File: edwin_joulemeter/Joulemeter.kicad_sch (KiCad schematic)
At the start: 57 parts, among them J1 XT60-M, J2 22035035, J3 22035035, J4 XT60-M, U1 INA240A3PWR, U3 MCP6286T-E/OT, U4 PADS131M04QPWRQ1

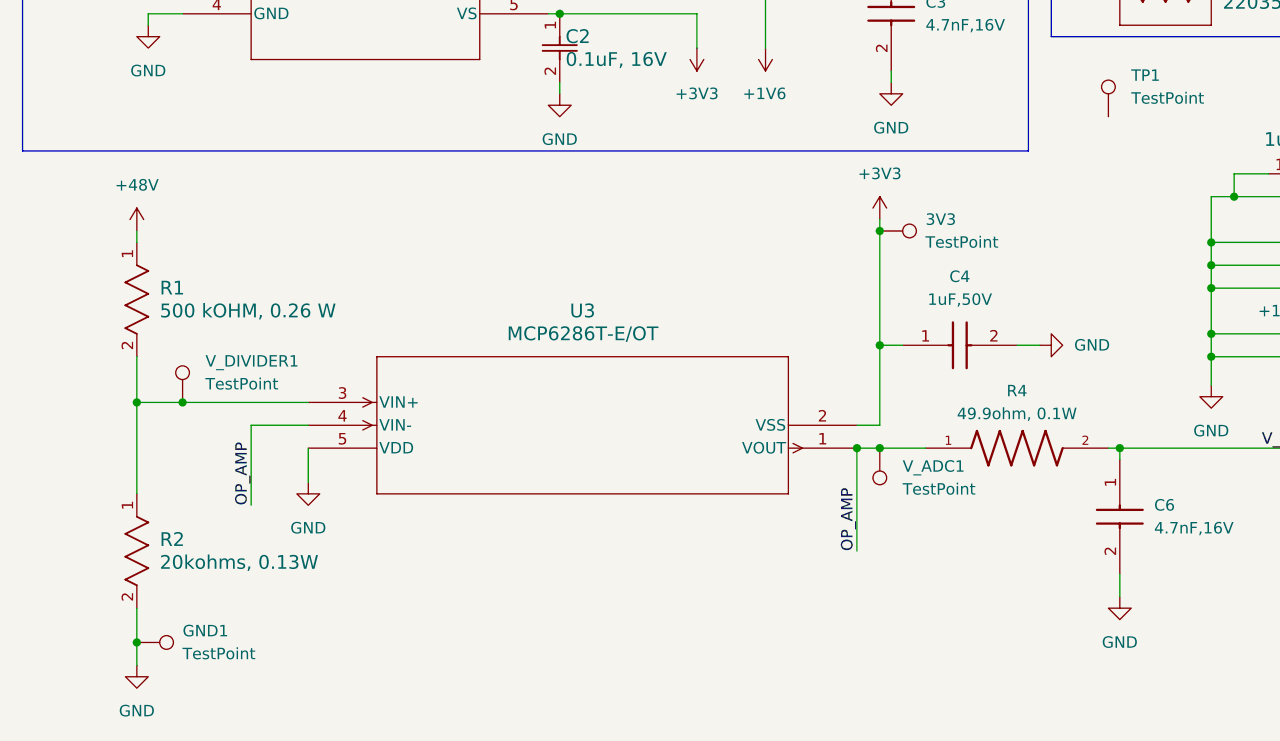
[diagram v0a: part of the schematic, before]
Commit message: jaj
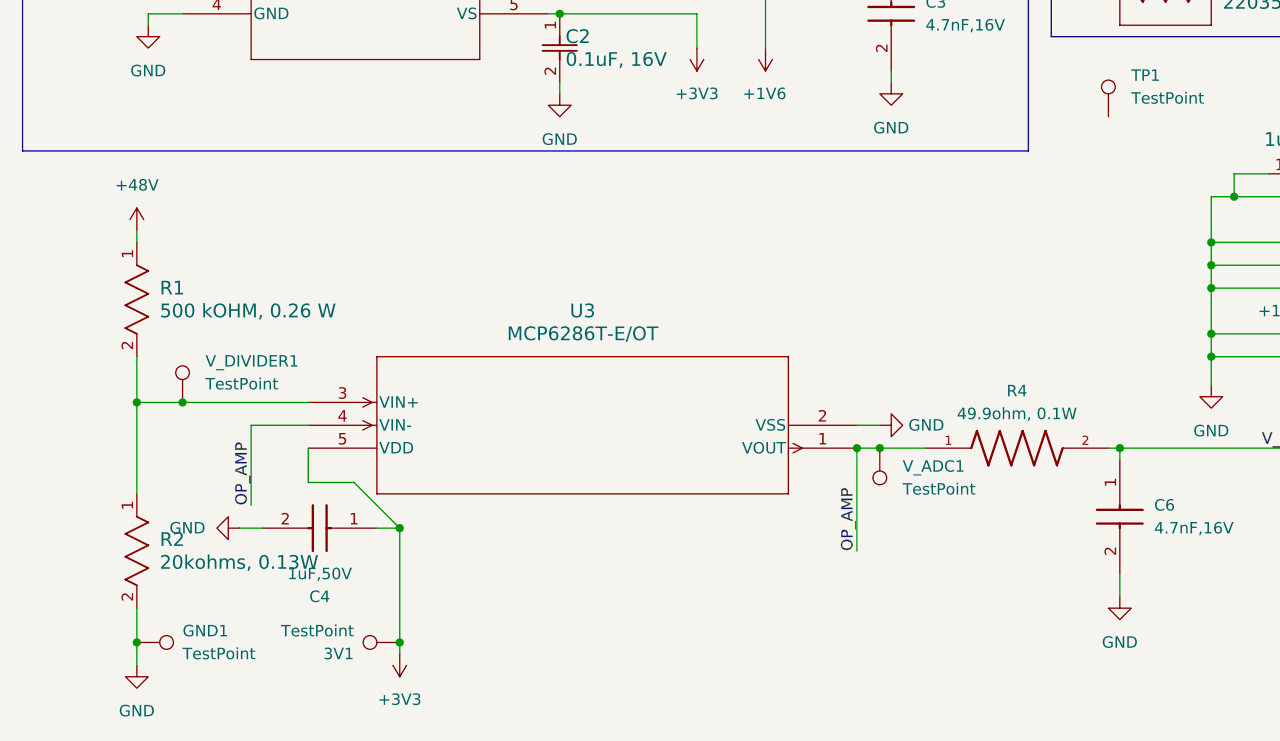
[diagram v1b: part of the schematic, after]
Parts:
- removed 3V3: TestPoint, TestPoint:TestPoint_Pad_1.5x1.5mm, symbol Connector:TestPoint
- added 3V1: TestPoint, TestPoint:TestPoint_Pad_1.5x1.5mm, symbol Connector:TestPoint
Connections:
- net +3V3: now also U3.5 (VDD), 3V1.1; no longer U3.2 (VSS)
- net GND: now also U3.2 (VSS); no longer U3.5 (VDD)
